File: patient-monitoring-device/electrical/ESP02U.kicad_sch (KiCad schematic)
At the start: 1 part, among them U1 ESP32-C3-WROOM-02U

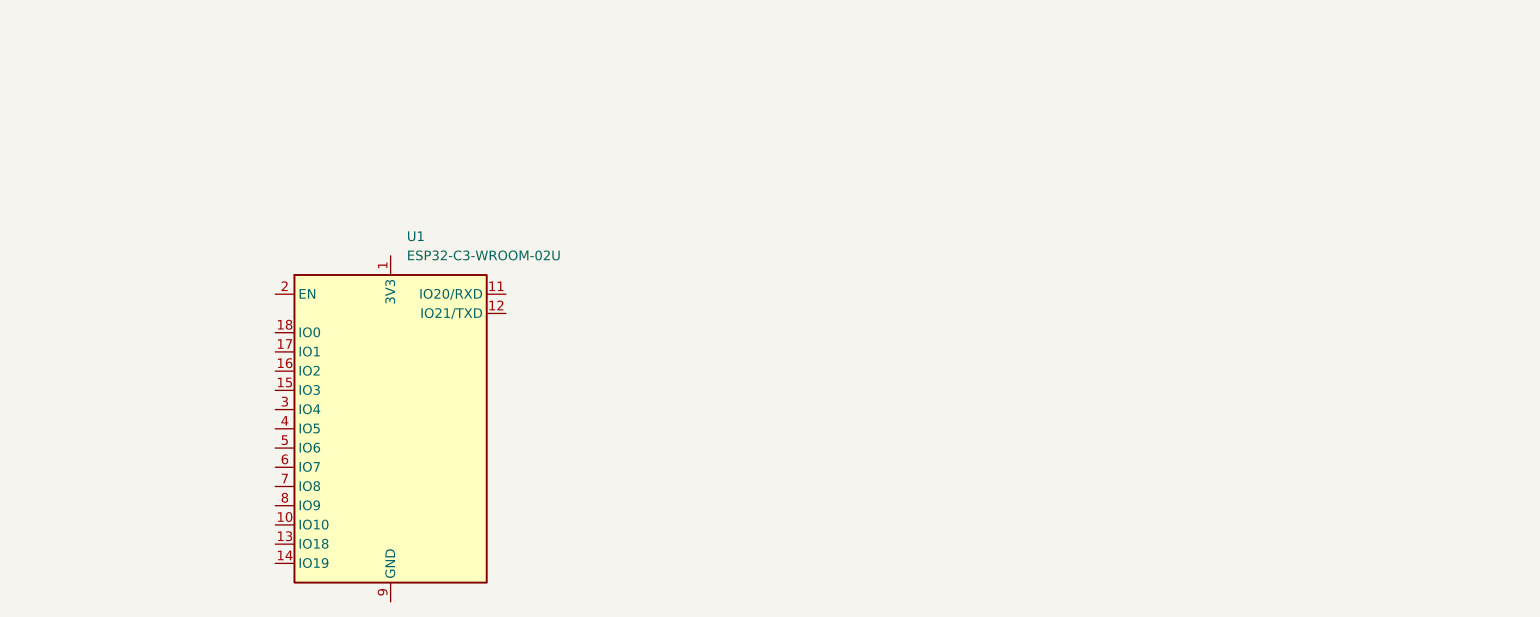
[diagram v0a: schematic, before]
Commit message: a few hours later
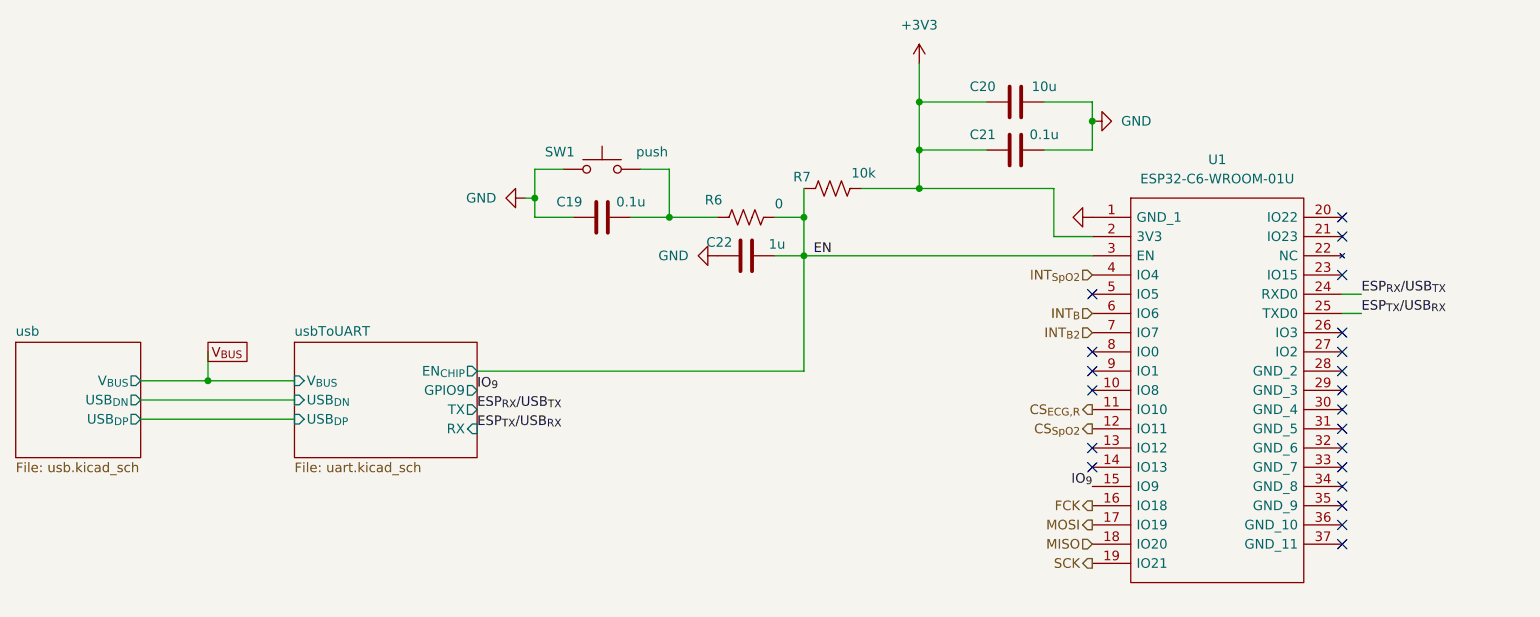
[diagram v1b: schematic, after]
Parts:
- added C19, C21: 0.1u, Capacitor_SMD:C_01005_0402Metric, symbol Device:C
- added C20: 10u, Capacitor_SMD:C_01005_0402Metric, symbol Device:C
- added C22: 1u, Capacitor_SMD:C_01005_0402Metric, symbol Device:C
- added R6: 0, Resistor_SMD:R_0201_0603Metric, symbol Device:R_US
- added R7: 10k, Resistor_SMD:R_0201_0603Metric, symbol Device:R_US
- added SW1: push, Button_Switch_SMD:SW_Push_SPST_NO_Alps_SKRK, symbol Switch:SW_Push
- U1: value ESP32-C3-WROOM-02U -> ESP32-C6-WROOM-01U; footprint RF_Module:ESP32-C3-WROOM-02U -> footprints:ESP32C6WROOM1UN8; symbol RF_Module:ESP32-C3-WROOM-02U -> symbols:ESP32-C6-WROOM-1U-N8; Description_1 (none) -> Multiprotocol Modules ESP32-C6 based module, supports Wi-Fi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; Height (none) -> 3.35; Manufacturer_Name (none) -> Espressif Systems; Manufacturer_Part_Number (none) -> ESP32-C6-WROOM-1U-N8; Mouser Part Number (none) -> 356-ESP32C6WROOM1UN8; Mouser Price/Stock (none) -> https://www.mouser.co.uk/ProductDetail/Espressif-Systems/ES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
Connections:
- net GND: now reaches U1.1 (GND_1)
- net GND: now also C19.1, C20.2, C21.2, C22.1, SW1.1
- net CS_{ECG,R}: now reaches U1.11 (IO10)
- net CS_{SpO2}: now reaches U1.12 (IO11)
- net IO_{9}: now reaches U1.15 (IO9)
- net FCK: now reaches U1.16 (IO18)
- net MOSI: now reaches U1.17 (IO19)
- net MISO: now reaches U1.18 (IO20)
- net at U1.9 (IO1): no longer U1.19 (GND)
- net +3V3: now reaches U1.2 (3V3)
- net +3V3: now also C20.1, C21.1, R7.1
- net EN: now reaches U1.3 (EN)
- net EN: now also C22.2, R6.2, R7.2
- net INT_{SpO2}: now reaches U1.4 (IO4)
- net INT_{B}: now reaches U1.6 (IO6)
- net INT_{B2}: now reaches U1.7 (IO7)
- new net: C19.2, R6.1, SW1.2
- new net ESP_{RX}/USB_{TX}: U1.24 (RXD0)
- new net ESP_{TX}/USB_{RX}: U1.25 (TXD0)
- new net SCK: U1.19 (IO21)
- no-connect marks 0 -> 21
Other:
- added sheet usb (usb.kicad_sch)
- added sheet usbToUART (uart.kicad_sch)
